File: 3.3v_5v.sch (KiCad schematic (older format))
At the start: 27 parts, among them J1 Jack-DC, SW1 SW_Push_SPDT, U1 AP1117-33, U6 MCP603-xCH

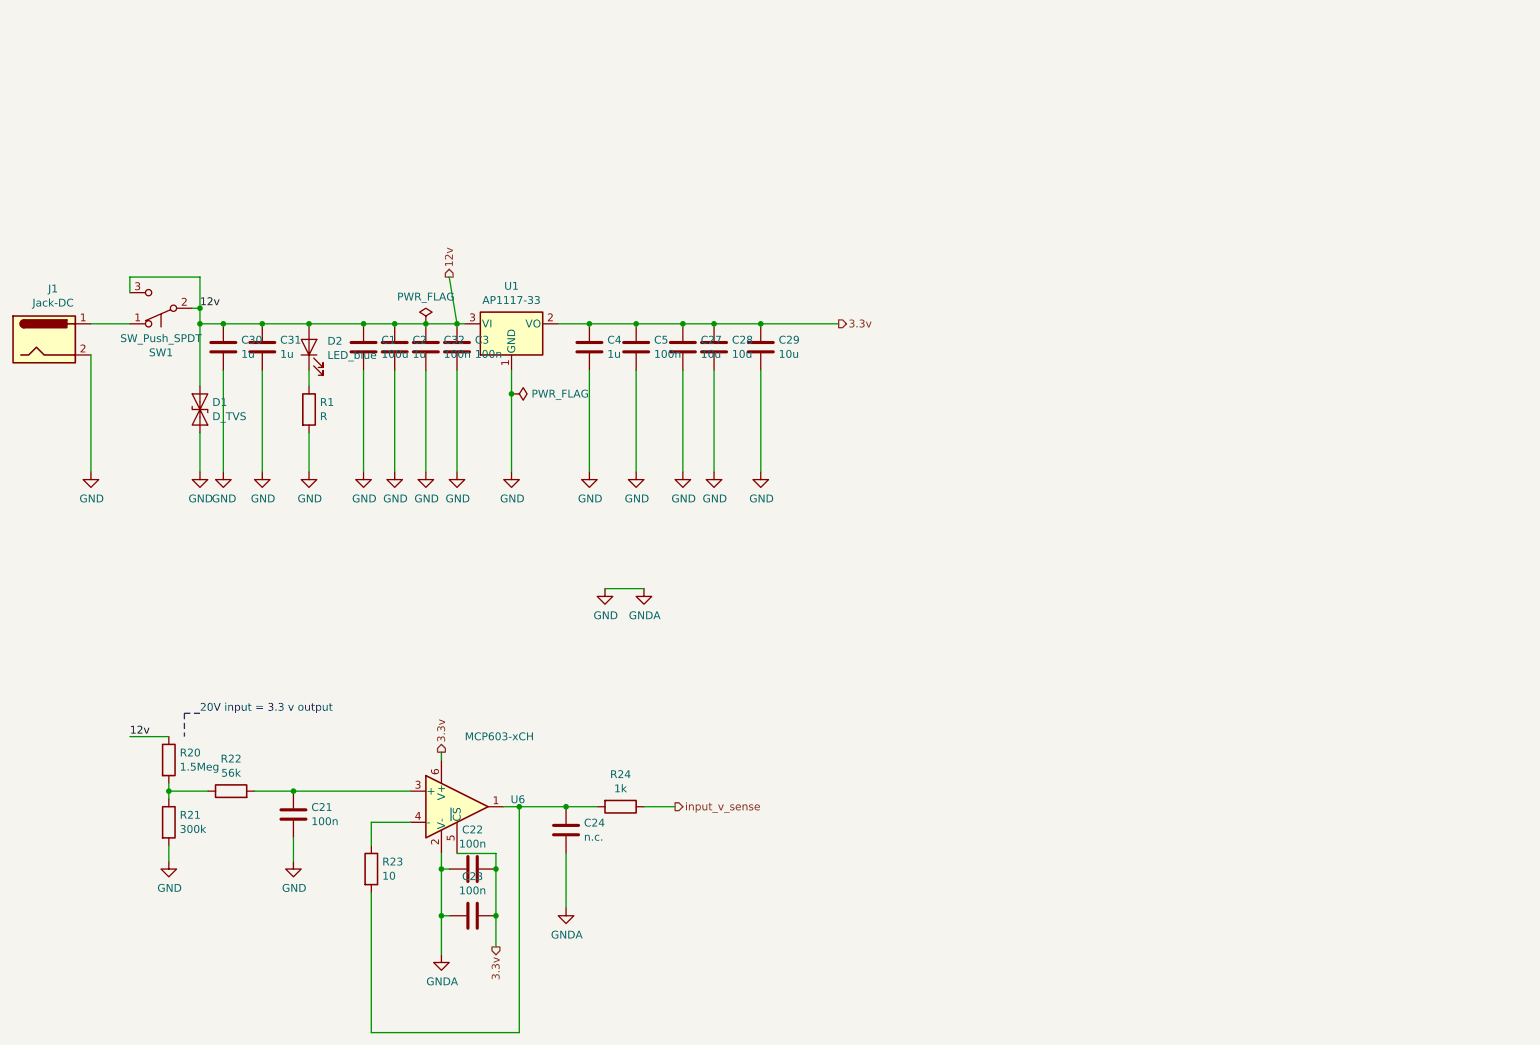
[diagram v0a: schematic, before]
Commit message: update front endu do termopary i przełącznika zasilającego
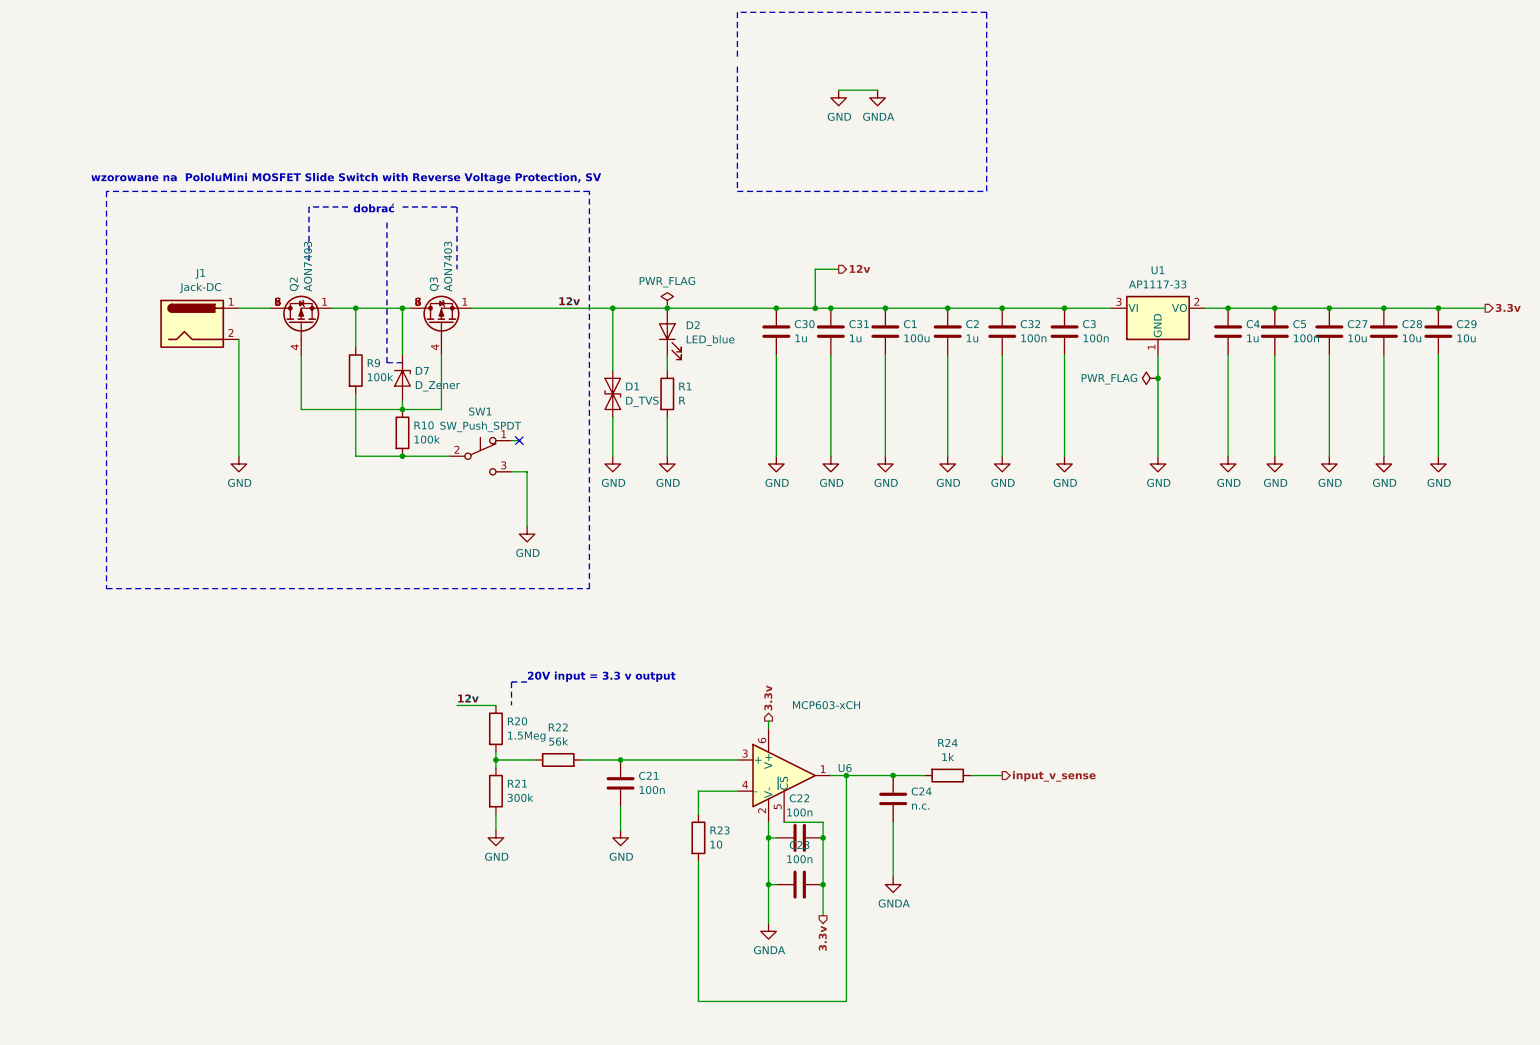
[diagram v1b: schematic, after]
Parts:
- added D7: D_Zener, Diode_SMD:D_0805_2012Metric_Castellated, symbol Device:D_Zener
- added Q2, Q3: AON7403, symbols:DFN_3X3_EP, symbol russian-nixies:AON7403
- added R10, R9: 100k, Resistor_SMD:R_0603_1608Metric, symbol Device:R
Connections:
- net 12v: now also Q3.1 (S), Q3.2 (S), Q3.3 (S); no longer SW1.2 (B), SW1.3 (C)
- net GND: now also SW1.3 (C)
- net at J1.1: now also Q2.5 (D), Q2.6 (D), Q2.7 (D), Q2.8 (D); no longer SW1.1 (A)
- new net: R10.2, R9.2, SW1.2 (B)
- new net: D7.1 (K), Q2.1 (S), Q2.2 (S), Q2.3 (S), Q3.5 (D), Q3.6 (D), Q3.7 (D), Q3.8 (D), R9.1
- new net: D7.2 (A), Q2.4 (G), Q3.4 (G), R10.1
- no-connect marks 0 -> 1
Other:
- note added: "dobrać"
- note added: "wzorowane na PololuMini MOSFET Slide Switch with Reverse Voltage Protection, SV\n"
- moved on the sheet: C1, C2, C21, C22, C23, C24, C27, C28, C29, C3, C30, C31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
